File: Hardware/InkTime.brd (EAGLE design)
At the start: 160 x 100 mm, 105 parts, among them IC1 BQ25180YBGR, IC2 DRV2605YZFR, IC3 BMA421, IC9 RT6160AWSC, J1 503480-2400, J2 TC2030-IDC, J4 KH-TYPE-C-16P, Q3 SI1308EDL-T1-GE3, U1 NRF52840_QF, U3 MAX17048G+T10, X1 32MHz, X2 32.768kHz

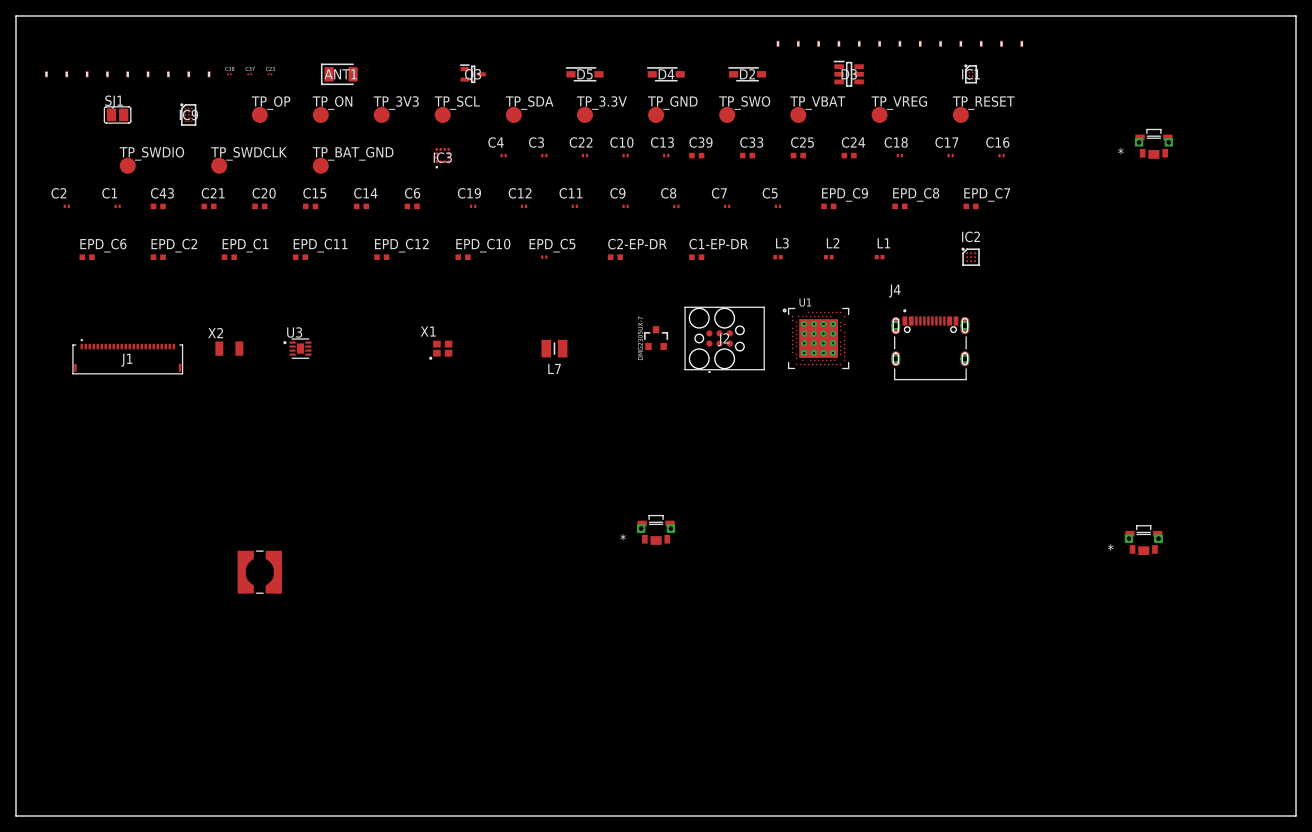
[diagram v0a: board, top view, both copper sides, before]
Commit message: Rezolvare issues
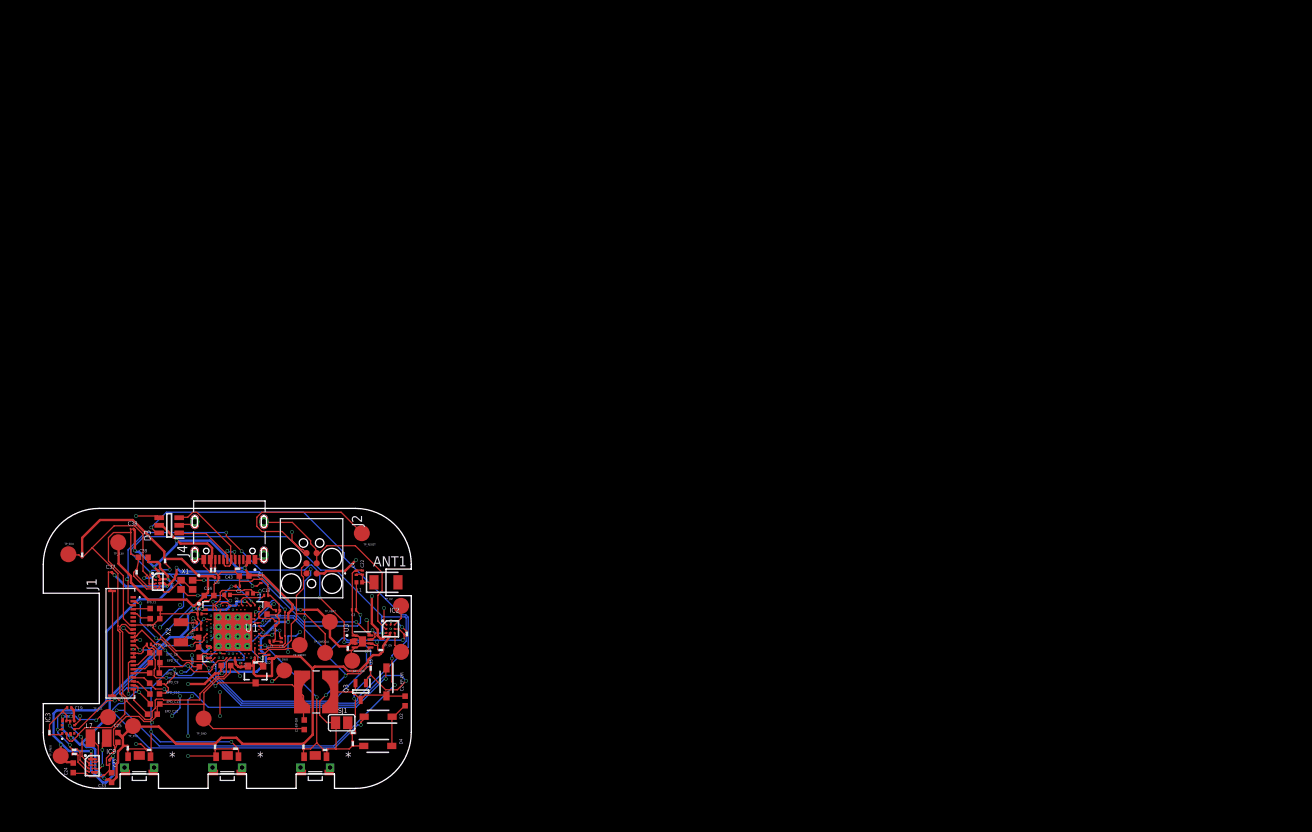
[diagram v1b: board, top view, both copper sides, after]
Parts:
- moved R2 148.0 mm to (7.30, 7.75), turned to 90 degrees
- moved R3 142.8 mm to (4.18, 10.4)
- moved R4 139.7 mm to (7.27, 8.28), turned to 90 degrees
- moved SW_ENT 139.3 mm to (26.4, 6.44), turned to 180 degrees
- moved R5 132.5 mm to (14.0, 8.49), turned to 180 degrees
- moved TP_VREG 130.0 mm to (5.59, 7.50)
- moved SW_UP 128.6 mm to (15.4, 6.44), turned to 180 degrees
- moved C24 123.5 mm to (7.15, 6.02), turned to 90 degrees
- moved R8 120.9 mm to (24.9, 8.64), turned to 180 degrees
- moved IC1 119.8 mm to (17.7, 29.3)
- moved EPD_C7 116.9 mm to (17.4, 19.2), turned to 180 degrees
- moved R2_USB 116.2 mm to (24.9, 30.8)
- moved R7 115.2 mm to (35.9, 8.64), turned to 180 degrees
- moved R18 112.1 mm to (8.27, 32.6)
- moved C25 111.9 mm to (12.7, 9.82), turned to 270 degrees
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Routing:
- net GND: track 0.00 -> 335.2 mm, vias 0 -> 15
- net 3V3: track 0.00 -> 190.6 mm, vias 0 -> 12
- net SCL: track 0.00 -> 135.7 mm, vias 0 -> 11
- net SDA: track 0.00 -> 107.5 mm, vias 0 -> 6
- net D-: track 0.00 -> 75.4 mm, vias 0 -> 2
- net VBUS: track 0.00 -> 68.9 mm, vias 0 -> 8
- net RESE: track 0.00 -> 61.1 mm, vias 0 -> 7
- net VREG: track 0.00 -> 56.2 mm, vias 0 -> 4
- net RESET: track 0.00 -> 53.1 mm, vias 0 -> 4
- net GDR: track 0.00 -> 50.6 mm, vias 0 -> 4
- net PREVGL: track 0.00 -> 43.2 mm, vias 0 -> 2
- net VBAT: track 0.00 -> 40.4 mm, vias 0 -> 4
- net ALERT: track 0.00 -> 39.9 mm, vias 0 -> 2
- net PREVGH: track 0.00 -> 36.0 mm, vias 0 -> 2
- net D+: track 0.00 -> 35.5 mm, vias 0 -> 2
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- added copper zone on layer 15, net GND
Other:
- board size 160 x 100 mm -> 46 x 35 mm
